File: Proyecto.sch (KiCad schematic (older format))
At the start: 52 parts, among them P1 CONN_01X03, P2 CONN_01X03, Q1 BC808-40, Q2 BC808-40, U1 MCP2515, U2 MCP2551-I/SN, U3 AMS1117, U4 ACS712, U5 ACS712

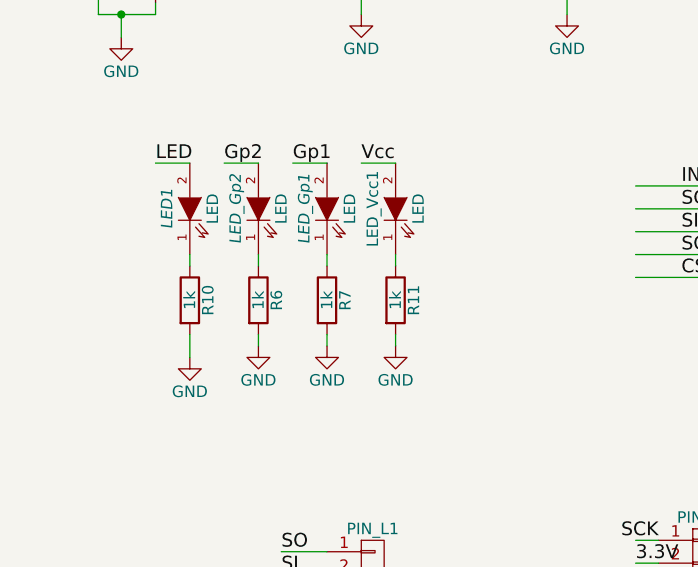
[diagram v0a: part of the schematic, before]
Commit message: fix pcb casa
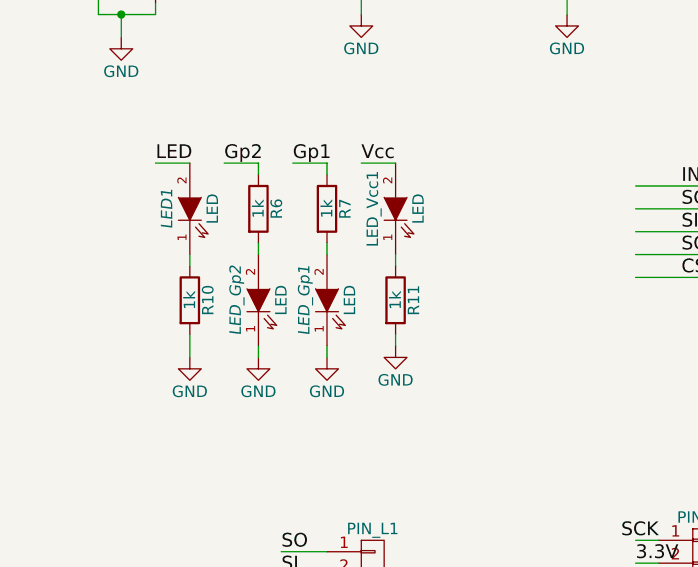
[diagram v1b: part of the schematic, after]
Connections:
- wire segments 198 -> 200
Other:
- moved on the sheet: LED_Gp1, LED_Gp2, R6, R7
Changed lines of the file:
@@
 LIBS:mylib
 LIBS:HK4100F
-LIBS:acs712
-LIBS:AMS1117
 LIBS:Proyecto-cache
 EELAYER 25 0
@@
 L LED LED_Gp2
 U 1 1 5777088E
+P 1600 3000
+F 0 "LED_Gp2" H 1600 3100 50  0000 C CIN
+F 1 "LED" H 1600 2900 50  0000 C CNN
+F 2 "LEDs:LED-3MM" H 1600 3000 50  0001 C CNN
+F 3 "" H 1600 3000 50  0000 C CNN
+	1    1600 3000
+	0    -1   -1   0
+$EndComp
+$Comp
+L R R6
+U 1 1 57770894
 P 1600 2600
-F 0 "LED_Gp2" H 1600 2700 50  0000 C CIN
-F 1 "LED" H 1600 2500 50  0000 C CNN
-F 2 "LEDs:LED-3MM" H 1600 2600 50  0001 C CNN
+F 0 "R6" V 1680 2600 50  0000 C CNN
+F 1 "1k" V 1600 2600 50  0000 C CNN
+F 2 "w_pth_resistors:RC05" V 1530 2600 50  0001 C CNN
 F 3 "" H 1600 2600 50  0000 C CNN
 	1    1600 2600
-	0    -1   -1   0
-$EndComp
-$Comp
-L R R6
-U 1 1 57770894
-P 1600 3000
-F 0 "R6" V 1680 3000 50  0000 C CNN
-F 1 "1k" V 1600 3000 50  0000 C CNN
-F 2 "w_pth_resistors:RC05" V 1530 3000 50  0001 C CNN
-F 3 "" H 1600 3000 50  0000 C CNN
-	1    1600 3000
 	1    0    0    -1
 $EndComp
@@
 L GND-RESCUE-Proyecto #PWR033
 U 1 1 5777089A
-P 1600 3200
-F 0 "#PWR033" H 1600 2950 50  0001 C CNN
-F 1 "GND" H 1600 3050 50  0000 C CNN
-F 2 "" H 1600 3200 50  0000 C CNN
-F 3 "" H 1600 3200 50  0000 C CNN
-	1    1600 3200
+P 1600 3250
+F 0 "#PWR033" H 1600 3000 50  0001 C CNN
+F 1 "GND" H 1600 3100 50  0000 C CNN
+F 2 "" H 1600 3250 50  0000 C CNN
+F 3 "" H 1600 3250 50  0000 C CNN
+	1    1600 3250
 	1    0    0    -1
 $EndComp
 Wire Wire Line
 	1450 2400 1600 2400
-Wire Wire Line
-	1600 2800 1600 2850
-Wire Wire Line
-	1600 3150 1600 3200
 Wire Wire Line
 	2950 6600 2850 6600
@@
 L LED LED_Gp1
 U 1 1 57770BB7
+P 1900 3000
+F 0 "LED_Gp1" H 1900 3100 50  0000 C CIN
+F 1 "LED" H 1900 2900 50  0000 C CNN
+F 2 "LEDs:LED-3MM" H 1900 3000 50  0001 C CNN
+F 3 "" H 1900 3000 50  0000 C CNN
+	1    1900 3000
+	0    -1   -1   0
+$EndComp
+$Comp
+L R R7
+U 1 1 57770BBD
 P 1900 2600
-F 0 "LED_Gp1" H 1900 2700 50  0000 C CIN
-F 1 "LED" H 1900 2500 50  0000 C CNN
-F 2 "LEDs:LED-3MM" H 1900 2600 50  0001 C CNN
+F 0 "R7" V 1980 2600 50  0000 C CNN
+F 1 "1k" V 1900 2600 50  0000 C CNN
+F 2 "w_pth_resistors:RC05" V 1830 2600 50  0001 C CNN
 F 3 "" H 1900 2600 50  0000 C CNN
 	1    1900 2600
-	0    -1   -1   0
-$EndComp
-$Comp
-L R R7
-U 1 1 57770BBD
-P 1900 3000
-F 0 "R7" V 1980 3000 50  0000 C CNN
-F 1 "1k" V 1900 3000 50  0000 C CNN
-F 2 "w_pth_resistors:RC05" V 1830 3000 50  0001 C CNN
-F 3 "" H 1900 3000 50  0000 C CNN
-	1    1900 3000
 	1    0    0    -1
 $EndComp
@@
 L GND-RESCUE-Proyecto #PWR034
 U 1 1 57770BC3
-P 1900 3200
-F 0 "#PWR034" H 1900 2950 50  0001 C CNN
-F 1 "GND" H 1900 3050 50  0000 C CNN
-F 2 "" H 1900 3200 50  0000 C CNN
-F 3 "" H 1900 3200 50  0000 C CNN
-	1    1900 3200
+P 1900 3250
+F 0 "#PWR034" H 1900 3000 50  0001 C CNN
+F 1 "GND" H 1900 3100 50  0000 C CNN
+F 2 "" H 1900 3250 50  0000 C CNN
+F 3 "" H 1900 3250 50  0000 C CNN
+	1    1900 3250
 	1    0    0    -1
 $EndComp
 Wire Wire Line
 	1750 2400 1900 2400
-Wire Wire Line
-	1900 2800 1900 2850
-Wire Wire Line
-	1900 3150 1900 3200
 Text Label 1450 2400 0    60   ~ 0
 Gp2
@@
 Text Label 2050 2400 0    60   ~ 0
 Vcc
-Wire Wire Line
-	1300 3150 1300 3250
 Wire Wire Line
 	5700 2300 6000 2300
@@
 Wire Wire Line
 	8150 3300 8150 3250
+Wire Wire Line
+	1300 3150 1300 3250
+Wire Wire Line
+	1900 3250 1900 3200
+Wire Wire Line
+	1600 3250 1600 3200
+Wire Wire Line
+	1900 2800 1900 2750
+Wire Wire Line
+	1600 2800 1600 2750
+Wire Wire Line
+	1600 2400 1600 2450
+Wire Wire Line
+	1900 2400 1900 2450
 $EndSCHEMATC
